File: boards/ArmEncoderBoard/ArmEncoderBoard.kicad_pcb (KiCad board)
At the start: 2 copper layers, 32.9 x 32.8 mm, 9 parts, among them J1 Conn_01x05, U2 AS5045B

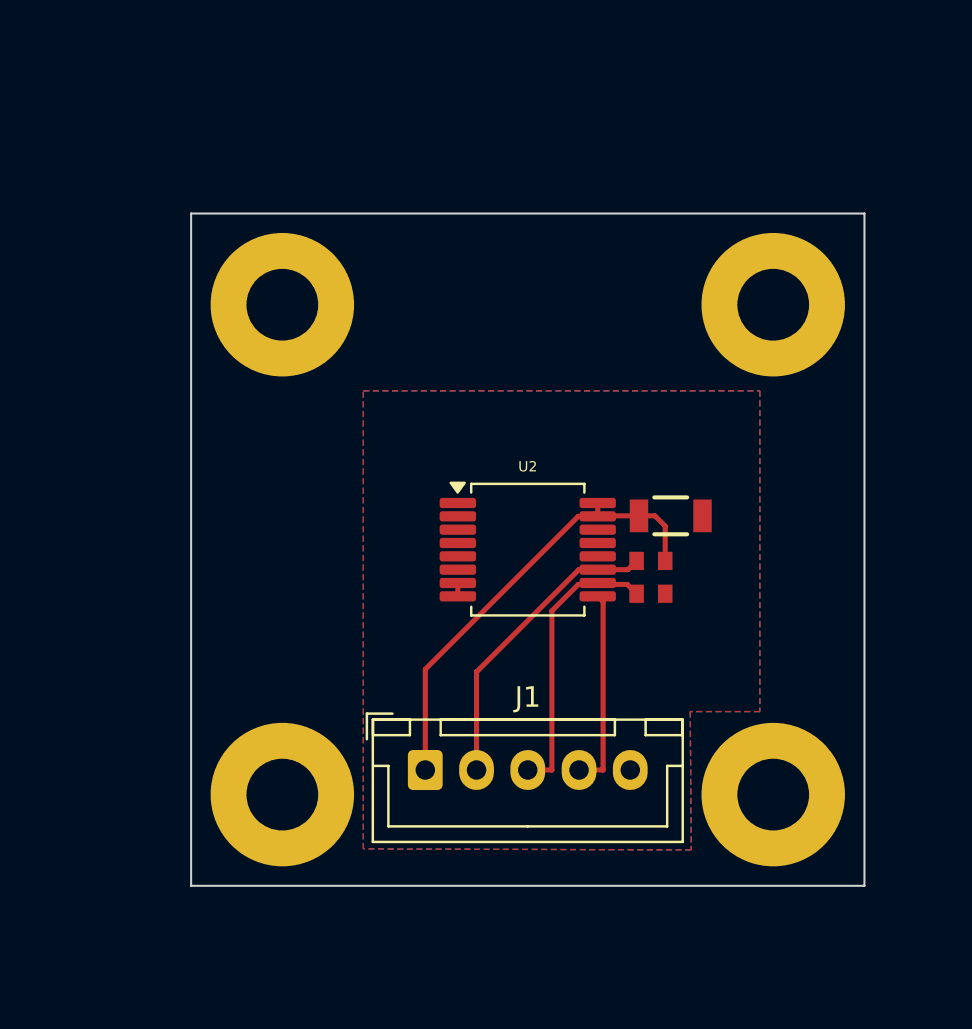
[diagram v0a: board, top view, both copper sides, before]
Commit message: Leg encoder board pre-final
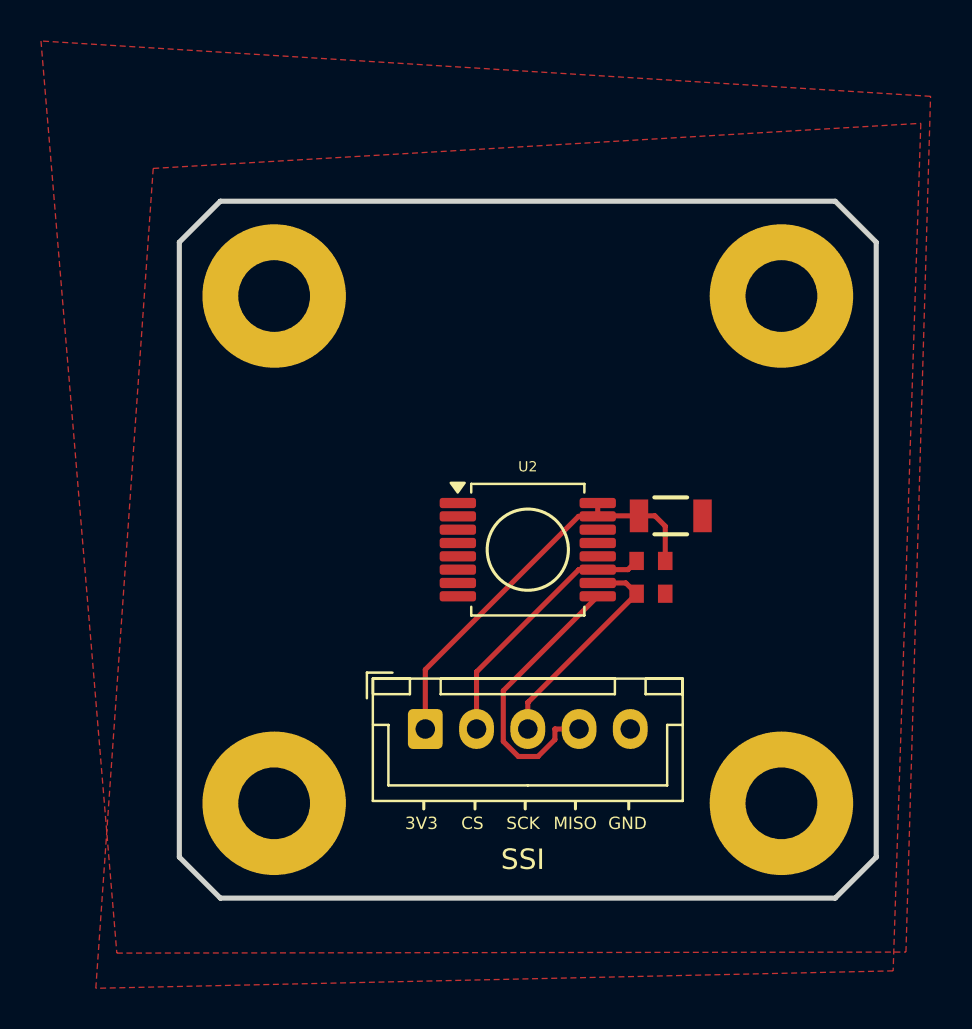
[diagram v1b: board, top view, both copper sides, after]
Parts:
- moved J1 2.00 mm to (133.7, 90.8)
- moved H2 0.58 mm to (151.1, 69.7)
- moved H4 0.58 mm to (151.1, 94.4)
- moved H1 0.58 mm to (126.4, 69.7)
- moved H3 0.58 mm to (126.4, 94.4)
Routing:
- net MISO: track 9.76 -> 13.8 mm
- net SCK: track 13.9 -> 10.9 mm
- net VIN: track 22.3 -> 20.3 mm
- net CS: track 14.8 -> 12.8 mm
- net GND: track 0.65 -> 0.00 mm
- removed copper zone on B.Cu, net GND
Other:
- board size 32.9 x 32.8 mm -> 34 x 34 mm
- board text added: "3V3"
- board text added: "CS"
- board text added: "GND"
- board text added: "MISO"
- board text added: "SCK"
- board text added: "SSI"
